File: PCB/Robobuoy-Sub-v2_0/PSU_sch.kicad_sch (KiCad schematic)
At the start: 69 parts, among them J201 Accu 1, J202 LoadbalanceAccu1, J203 LoadbalanceAccu2, J204 CHARGE/ON-OFF, J205 Accu 2, J206 ESCSB, J207 ESCBB, Q201 AO3400A, Q202 AO3400A, Q203 AO3400A, Q204 AO3400A, Q205 AO3400A, Q206 AO3400A, Q207 AO3400A, Q208 AO3400A, SW201 On/Off, U201 TPS5430DDAR, U202 SN74LV1T34DBV, U203 SN74LV1T34DBV, U204 TLV61046ADB

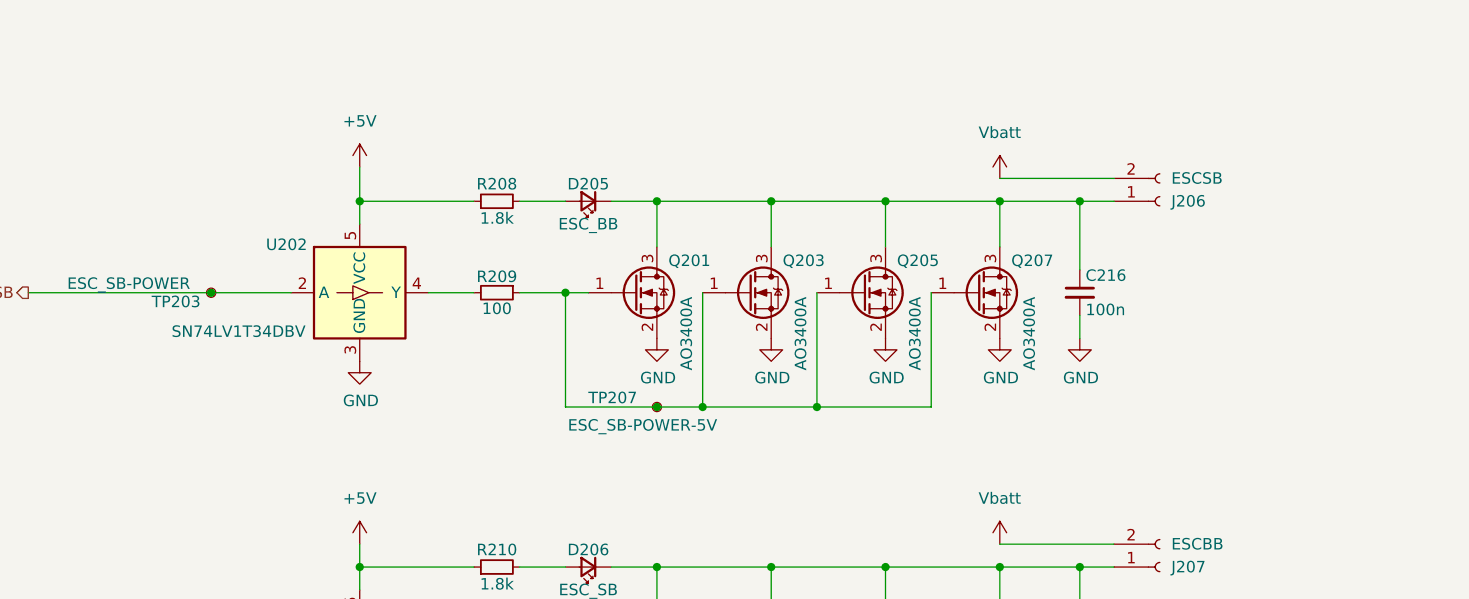
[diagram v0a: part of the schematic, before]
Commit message: Pc programm starting to code
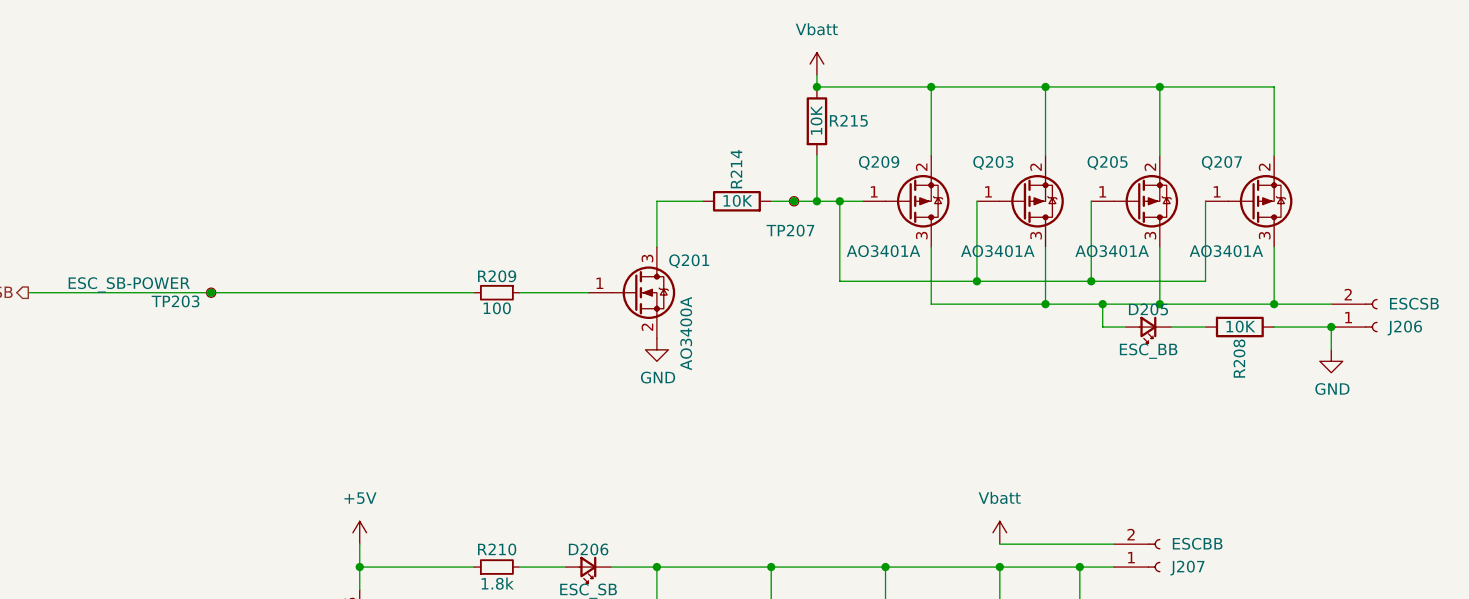
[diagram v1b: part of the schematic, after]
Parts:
- removed C216: 100n, A_Device:C_0603, symbol Device:C_Small
- removed Q203, Q205, Q207: AO3400A, Package_TO_SOT_SMD:SOT-23, symbol Transistor_FET:2N7002
- removed R208: 1.8k, A_Device:R_0603, symbol Device:R_Small
- removed U202: SN74LV1T34DBV, Package_TO_SOT_SMD:SOT-23-5, symbol Logic_LevelTranslator:SN74LV1T34DBV
- added Q203, Q205, Q207, Q209: AO3401A, Package_TO_SOT_SMD:SOT-23, symbol Transistor_FET:AO3401A
- added R208, R214, R215: 10K, A_Device:R_0603, symbol Device:R
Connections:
- net GND: now also J206.1 (Pin_1), R208.1
- net PWR_ESC_SB: now also R209.2
- net Vbatt: now also Q203.2 (S), Q205.2 (S), Q207.2 (S), Q209.2 (S), R215.1; no longer J206.2 (Pin_2)
- net at Q201.1 (G), R209.1: no longer TP207.1
- net at D205.2 (A): now also J206.2 (Pin_2), Q203.3 (D), Q205.3 (D), Q207.3 (D), Q209.3 (D)
- new net: Q201.3 (D), R214.1
- new net: D205.1 (K), R208.2
- new net: Q203.1 (G), Q205.1 (G), Q207.1 (G), Q209.1 (G), R214.2, R215.2, TP207.1
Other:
- moved on the sheet: D205, J206, TP207
